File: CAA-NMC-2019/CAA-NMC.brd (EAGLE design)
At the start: 100.2 x 100.4 mm, 28 parts, among them IC1 ATTINY85-20SU, J1 M20-9980346

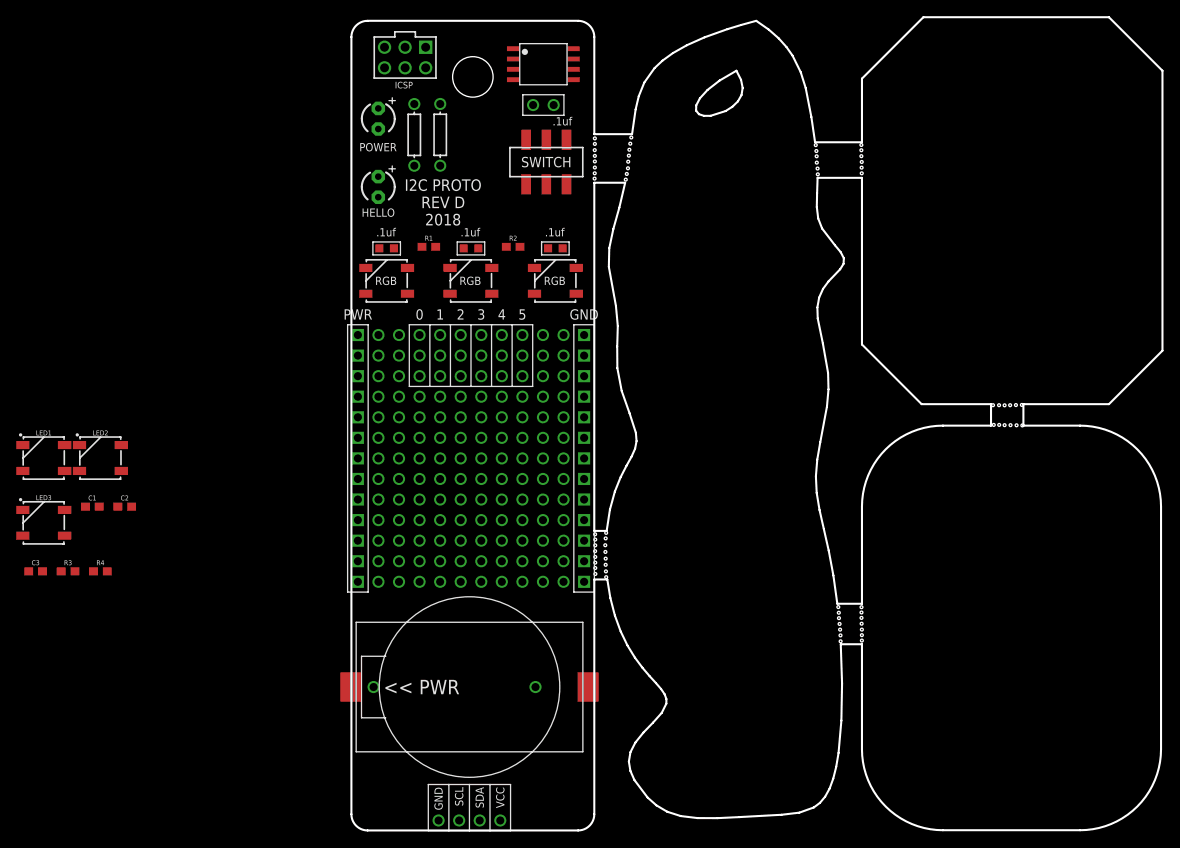
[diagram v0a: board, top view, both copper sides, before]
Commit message: Roll back to boring profile
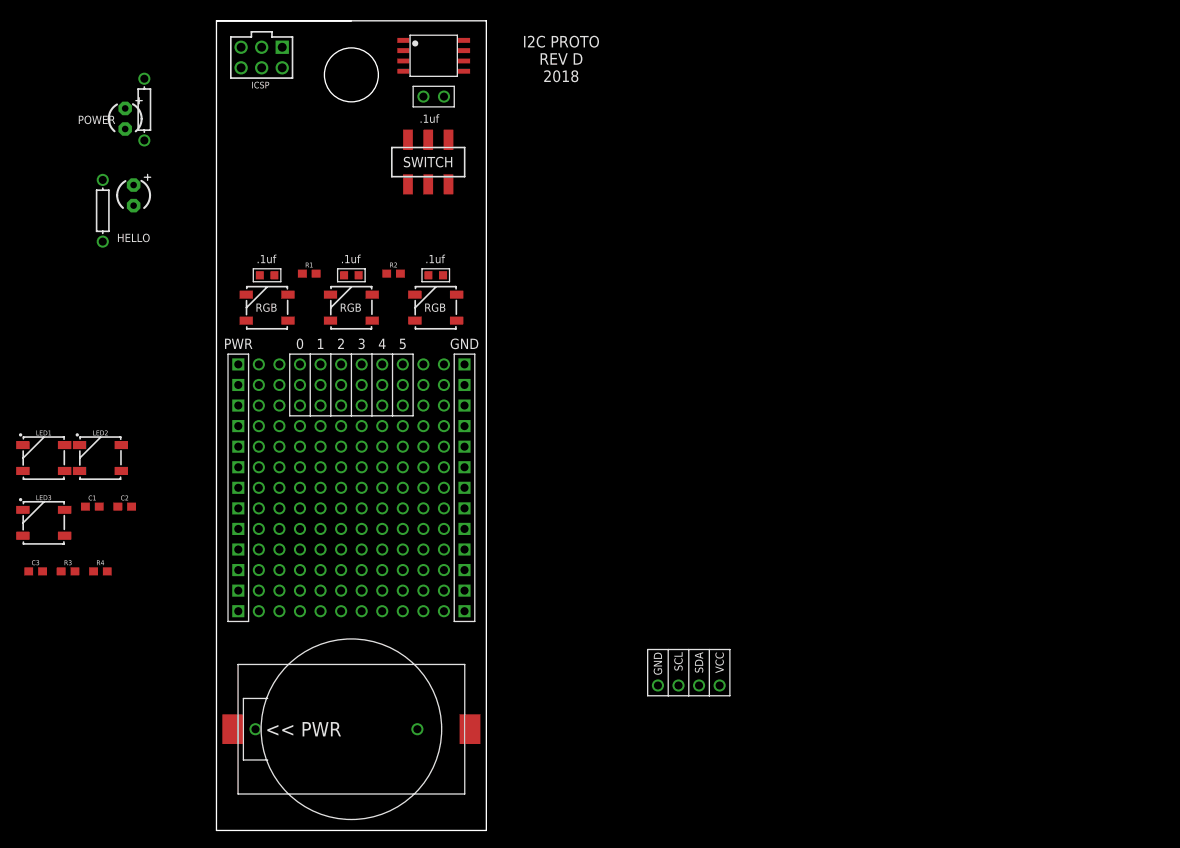
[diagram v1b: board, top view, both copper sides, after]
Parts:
- moved U$127 42.7 mm to (-30.7, 76.5)
- moved U$126 33.5 mm to (-25.6, 89.0)
- moved U$71 31.8 mm to (37.9, 17.9)
- moved U$72 31.8 mm to (42.9, 17.9)
- moved U$73 31.8 mm to (40.4, 17.9)
- moved U$74 31.8 mm to (45.5, 17.9)
- moved POWER 31.3 mm to (-27.9, 87.9)
- moved HELLO 30.2 mm to (-26.9, 78.4)
- moved J1 17.7 mm to (-11.1, 92.9)
- moved U$2 15.5 mm to (0.00, 12.5)
- moved U$3 15.5 mm to (0.00, 12.5)
- moved U$1 15.2 mm to (0.00, 27.1)
- moved D3 15.1 mm to (10.4, 64.6)
- moved D1 15.1 mm to (-10.4, 64.6)
- moved D2 15.1 mm to (-0.01, 64.6)
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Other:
- board size 100.2 x 100.4 mm -> 33.3 x 100 mm
